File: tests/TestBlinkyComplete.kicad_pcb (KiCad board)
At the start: 2 copper layers, 48 x 12 mm, 16 parts, among them J1 COM-15111, J2 PinHeader1.27 Shrouded 2x5, U1 LD1117S33TR, U2 STM32F103xxT6

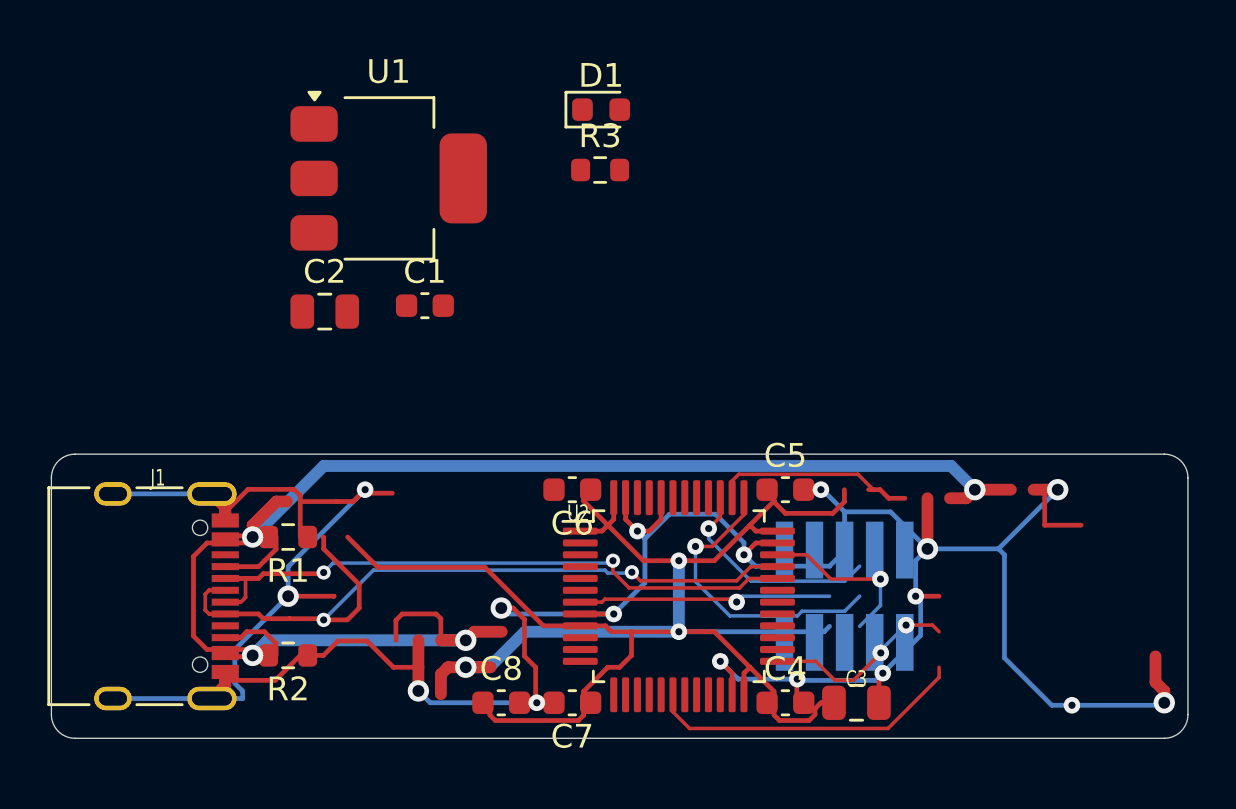
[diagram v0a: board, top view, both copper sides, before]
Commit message: more save filtering
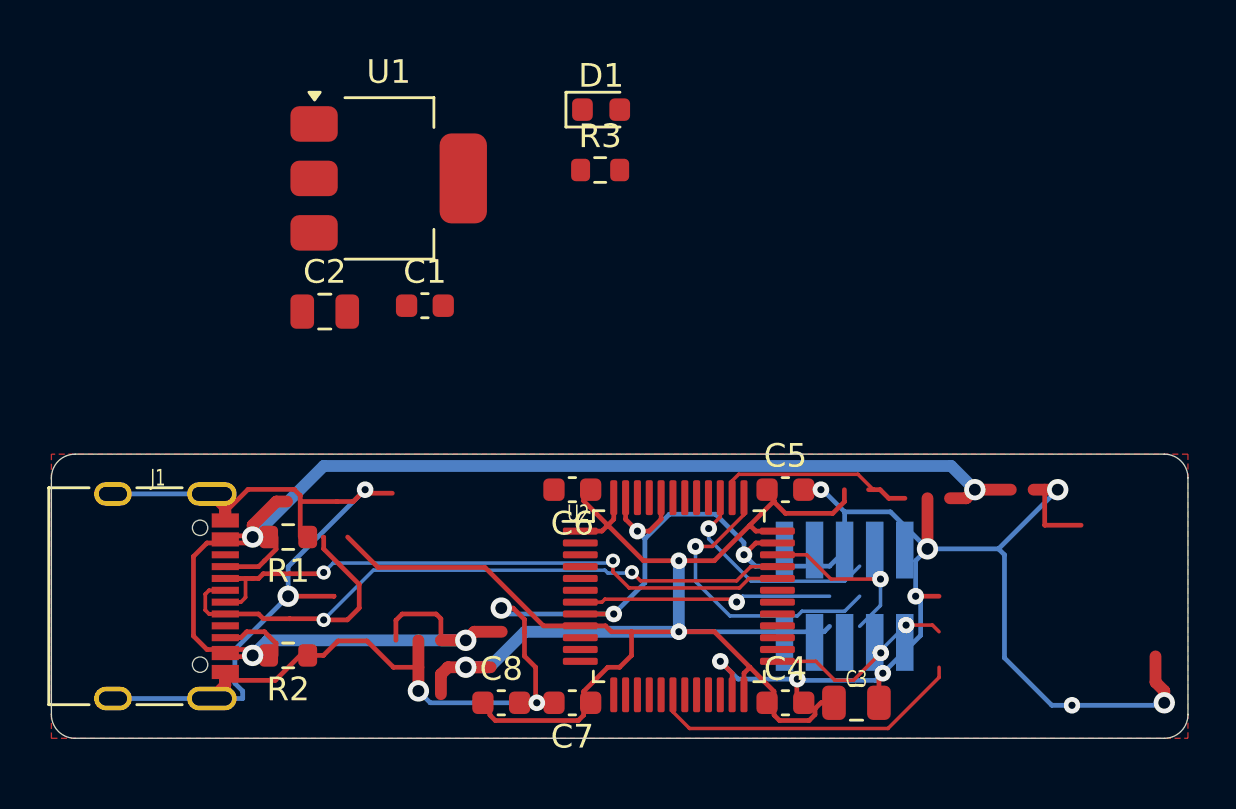
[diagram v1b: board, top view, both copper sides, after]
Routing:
- added copper zone on F.Cu, net gnd
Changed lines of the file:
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@@
 		(net 20)
 	)
+	(zone
+		(net 1)
+		(net_name "gnd")
+		(layer "F.Cu")
+		(hatch edge 0.5)
+		(connect_pads
+			(clearance 0.5)
+		)
+		(min_thickness 0.25)
+		(filled_areas_thickness no)
+		(fill
+			(thermal_gap 0.5)
+			(thermal_bridge_width 0.5)
+		)
+		(polygon
+			(pts
+				(xy 134 42) (xy 134 54) (xy 182 54) (xy 182 42)
+			)
+		)
+	)
 )
